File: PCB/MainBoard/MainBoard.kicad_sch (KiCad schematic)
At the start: 17 parts, among them J1 PiPowerSwitch, J2 Pi_Zero, J3 I2C0, J4 JMD0.96C, J5 WS2812, J6 Extra_Keys, J8 JoyStick_Or_I2C1, SW1 SPI_SW, SW2 RotaryEncoder_Switch, U1 Pico

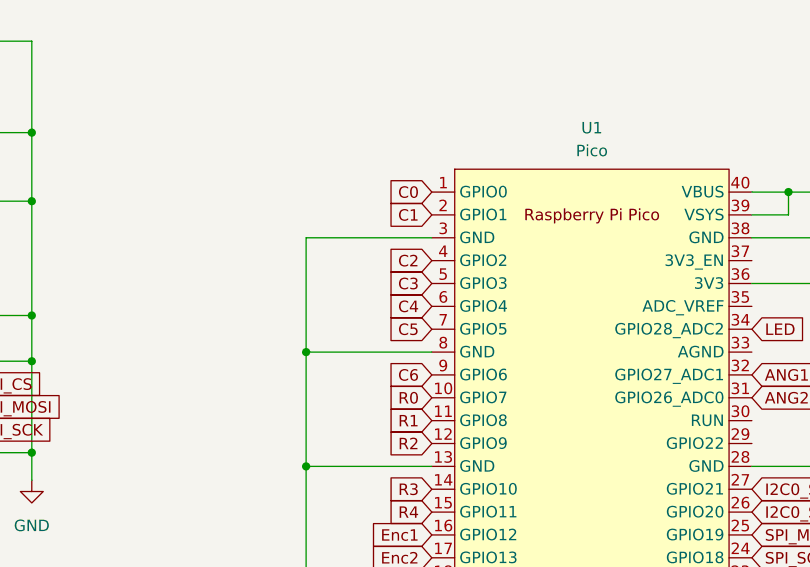
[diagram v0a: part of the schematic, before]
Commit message: Whatever
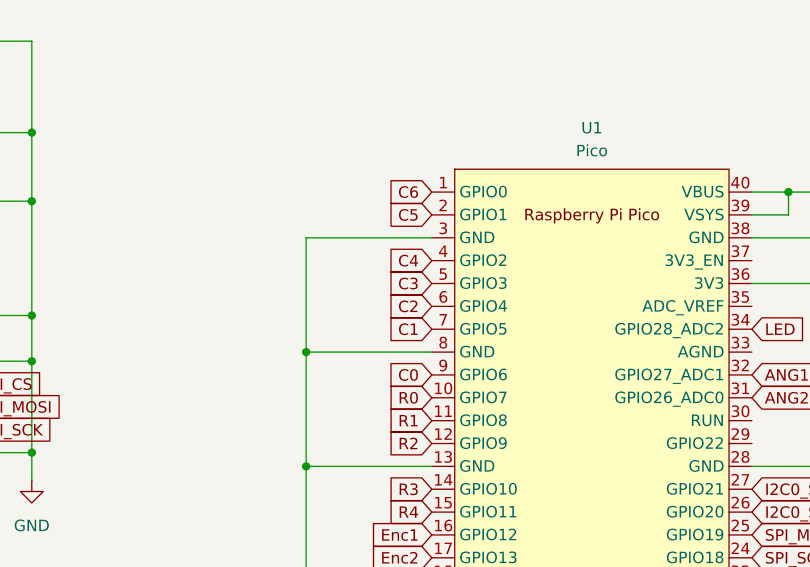
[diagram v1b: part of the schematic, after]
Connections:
- net C0: now also U1.9 (GPIO6); no longer U1.1 (GPIO0)
- net C1: now also U1.7 (GPIO5); no longer U1.2 (GPIO1)
- net C2: now also U1.6 (GPIO4); no longer U1.4 (GPIO2)
- net C4: now also U1.4 (GPIO2); no longer U1.6 (GPIO4)
- net C5: now also U1.2 (GPIO1); no longer U1.7 (GPIO5)
- net C6: now also U1.1 (GPIO0); no longer U1.9 (GPIO6)
